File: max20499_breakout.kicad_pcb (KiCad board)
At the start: 2 copper layers, 70 x 26.5 mm, 36 parts, among them J1 Conn_01x01, J2 Conn_01x01, J3 Conn_01x04, J4 Conn_01x01, J5 Conn_01x01, U1 MAX20499

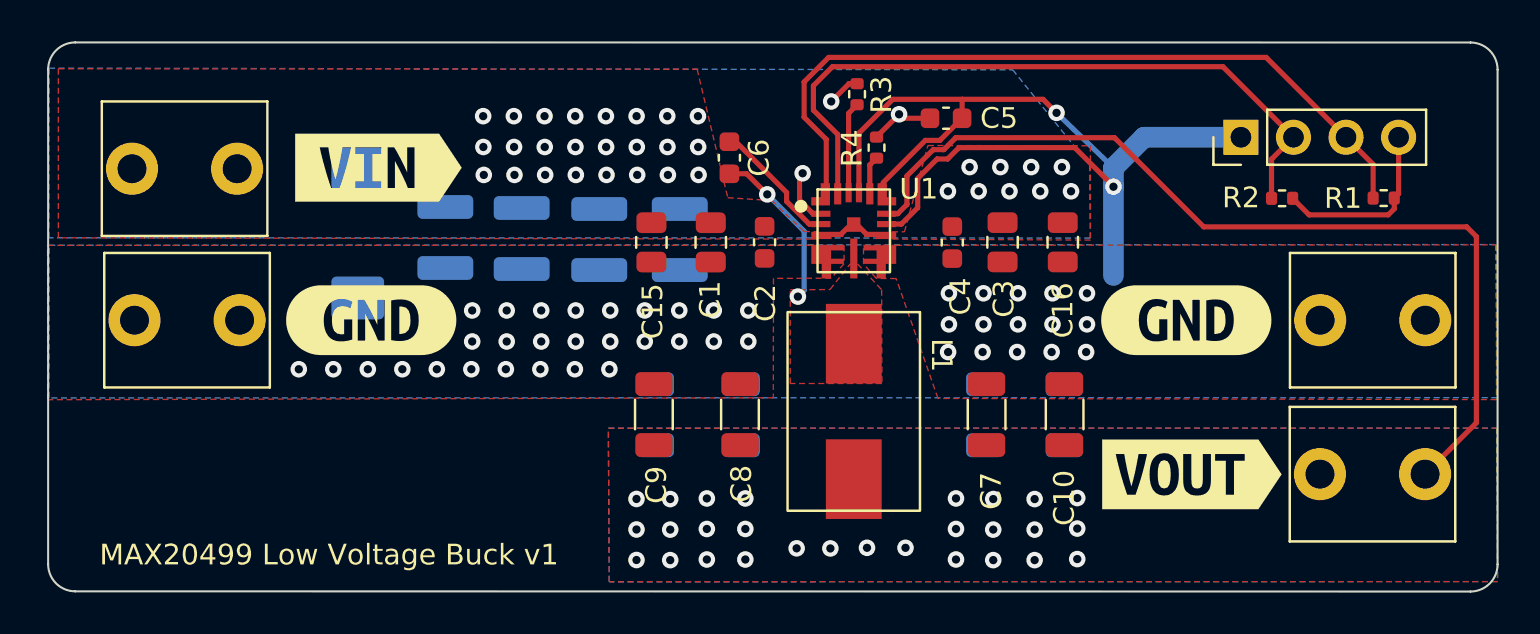
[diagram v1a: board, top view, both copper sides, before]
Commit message: lil' silkscreen tweak. regenerated gerbers
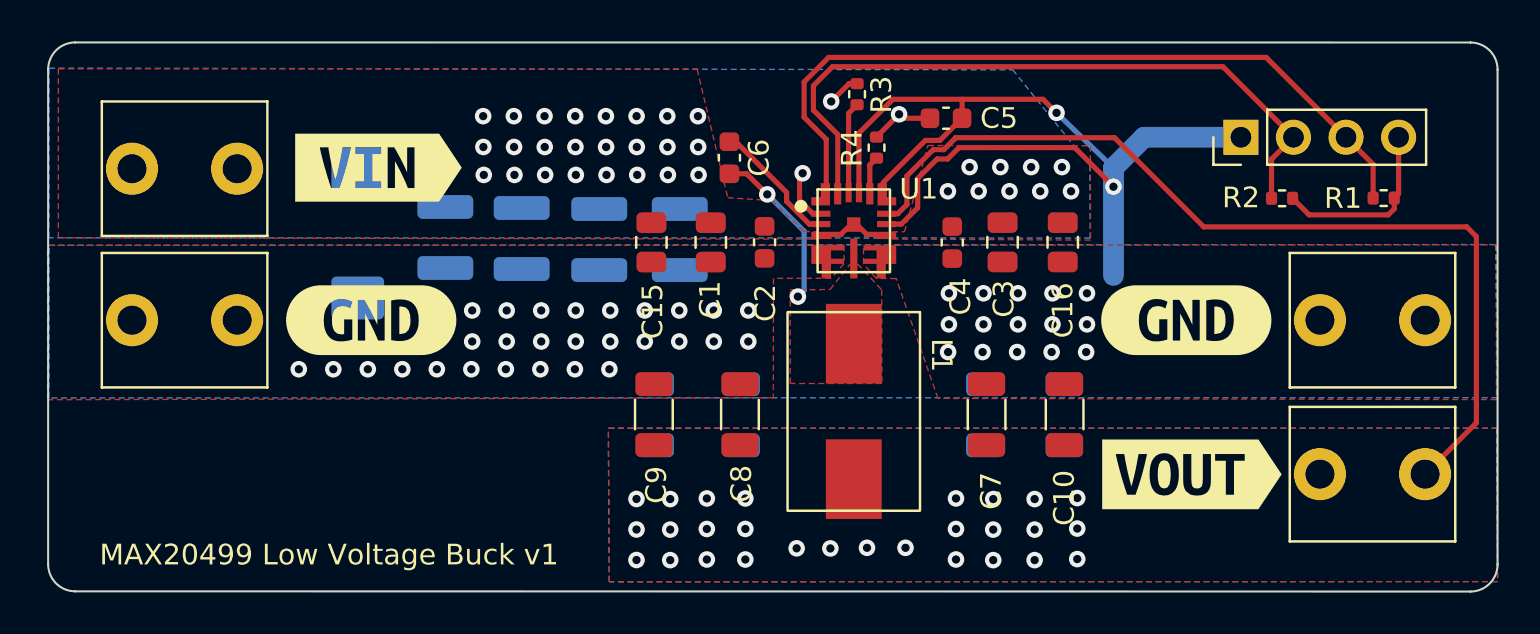
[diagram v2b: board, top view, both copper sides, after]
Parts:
- moved J1 0.12 mm to (99.2, 97.6)
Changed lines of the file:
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@@
   (net 10 "/SCL")
   (footprint "low_voltage_reg:63862-1" (layer "F.Cu")
-    (at 99.31 97.6)
+    (at 99.19 97.6)
     (property "Sheetfile" "max20499_breakout.kicad_sch")
     (property "Sheetname" "")
@@
   )
   (footprint "low_voltage_reg:63862-1" (layer "F.Cu")
-    (at 156.61 97.6)
-    (property "Sheetfile" "max20499_breakout.kicad_sch")
-    (property "Sheetname" "")
+    (at 156.6 97.6)
+    (property "Sheetfile" "max20499_breakout.kicad_sch")
+    (property "Sheetname" "")
